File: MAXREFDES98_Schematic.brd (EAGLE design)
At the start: 87.8 x 25.4 mm, 34 parts, among them U1 MB110S-TP, U2 MB110S-TP, U3 MAX5969AETB+

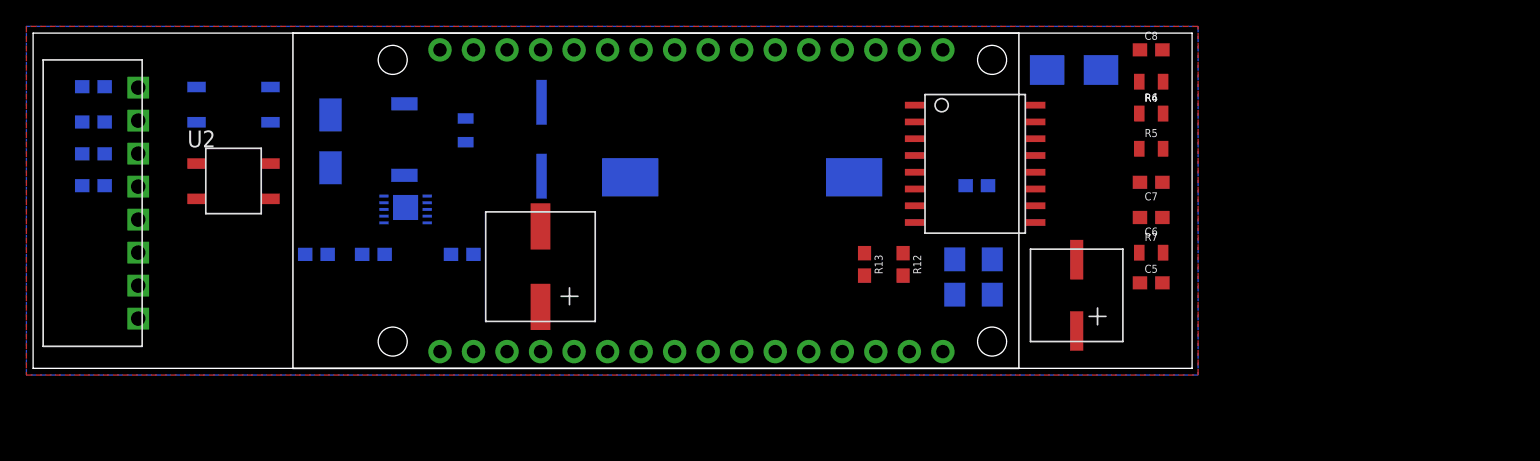
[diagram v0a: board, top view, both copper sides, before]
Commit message: Placement
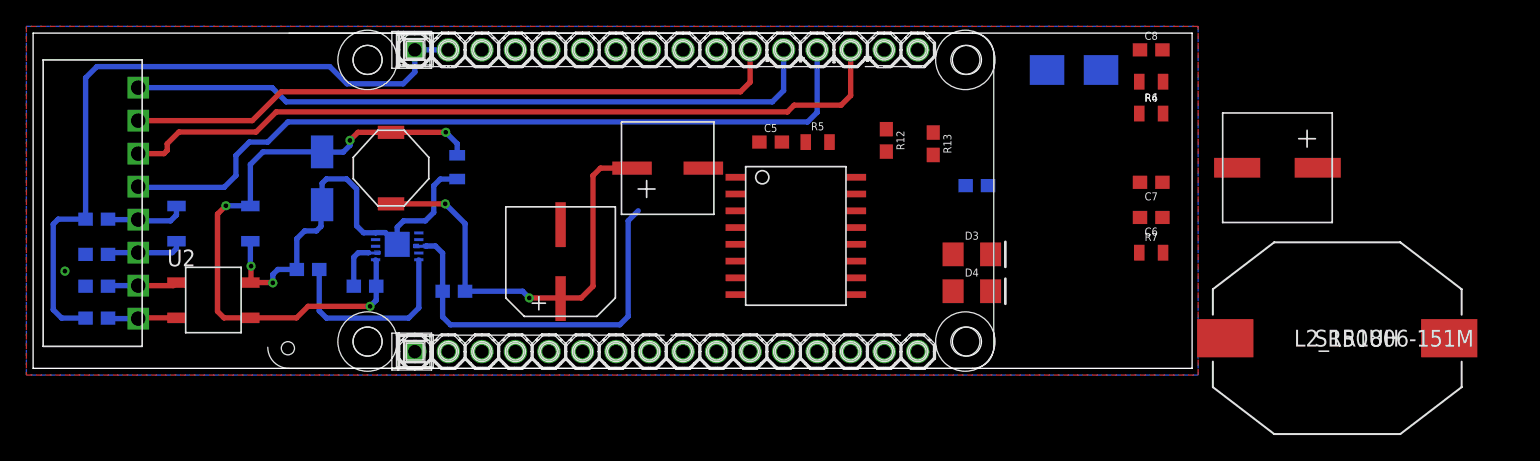
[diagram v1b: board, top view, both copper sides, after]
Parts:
- moved C3 57.0 mm to (94.6, 14.9), turned to 90 degrees
- moved L2_150UH 46.7 mm to (98.8, 2.29), flipped to the top, turned to 0 degrees
- moved C4 35.2 mm to (44.6, 18.7), turned to 270 degrees
- moved C5 30.7 mm to (55.9, 17.1)
- moved U$2 25.5 mm to (17.8, 25.4), flipped to the bottom, turned to 180 degrees
- moved R5 25.3 mm to (59.4, 17.1)
- moved U$1 14.6 mm to (57.8, 10.0)
- moved C2 11.5 mm to (35.8, 3.94), flipped to the top
- moved R13 10.5 mm to (68.2, 17.0)
- moved R10 10.0 mm to (4.83, 8.64)
- moved R9 10.0 mm to (4.83, 6.22)
- moved R11 10.0 mm to (4.83, 3.81)
- moved R8 10.0 mm to (4.83, 11.3)
- moved R12 9.48 mm to (64.6, 17.3)
- moved U1 9.14 mm to (10.2, 12.7)
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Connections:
- new net VDD_L: C2.PLUS, C4.PLUS, C5.1, L1.P$2, R3.2, R7.1, U$1.11
- net RD+: now also CONN.1; no longer CONN.5
- net RD-: now also CONN.2; no longer CONN.6
- net RECT1_IN_MINUS: now also CONN.6; no longer CONN.2
- net RECT1_IN_PLUS: now also CONN.5; no longer CONN.1
- net RECT2_IN_MINUS: now also CONN.7; no longer CONN.3
- net RECT2_IN_PLUS: now also CONN.8; no longer CONN.4
- net TD+: now also CONN.3; no longer CONN.7
- net TD-: now also CONN.4; no longer CONN.8
- net VDD: no longer C2.PLUS, C4.PLUS, C5.1, L1.P$2, R3.2, R7.1, U$1.11
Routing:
- net TD+: track 0.00 -> 59.6 mm
- net TD-: track 0.00 -> 59.4 mm
- net 5V_OUT: track 0.00 -> 52.9 mm
- net RD+: track 0.00 -> 52.8 mm
- net RD-: track 0.00 -> 50.0 mm
- net VDD: track 0.00 -> 47.3 mm, vias 0 -> 4
- net VSS_EP: track 0.00 -> 33.6 mm, vias 0 -> 2
- net VDD_L: track 0.00 -> 33.3 mm, vias 0 -> 2
- net PG_EN/SS_INH: track 0.00 -> 29.2 mm
- net CLS: track 0.00 -> 14.9 mm
- net RECT1_IN_PLUS: track 0.00 -> 6.13 mm
- net RECT1_IN_MINUS: track 0.00 -> 6.06 mm
- net RECT2_IN_MINUS: track 0.00 -> 5.30 mm
- net RECT2_IN_PLUS: track 0.00 -> 5.25 mm
- net DET: track 0.00 -> 3.44 mm
- added copper zone on layer 16, net DET
- added copper zone on layer 16, net PG_EN/SS_INH
